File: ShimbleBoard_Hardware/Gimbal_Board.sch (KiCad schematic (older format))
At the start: 84 parts, among them Q1 Q_NMOS_GDS, Q2 Q_NMOS_GDS, Q3 Q_NMOS_GDS, Q4 Q_NMOS_GDS, Q5 Q_NMOS_GDS, Q6 Q_NMOS_GDS, Q7 Q_NMOS_GDS, Q8 Q_NMOS_GDS, SW1 SW_Push, SW10 SW_SPDT, SW2 SW_Push, SW3 SW_Push, SW4 SW_Push, SW5 SW_Push, SW6 SW_Push, SW7 SW_Push, SW8 SW_Push, SW9 SW_Push, U1 TM4C129E_Launchpad, U2 OKI, U3 OKI

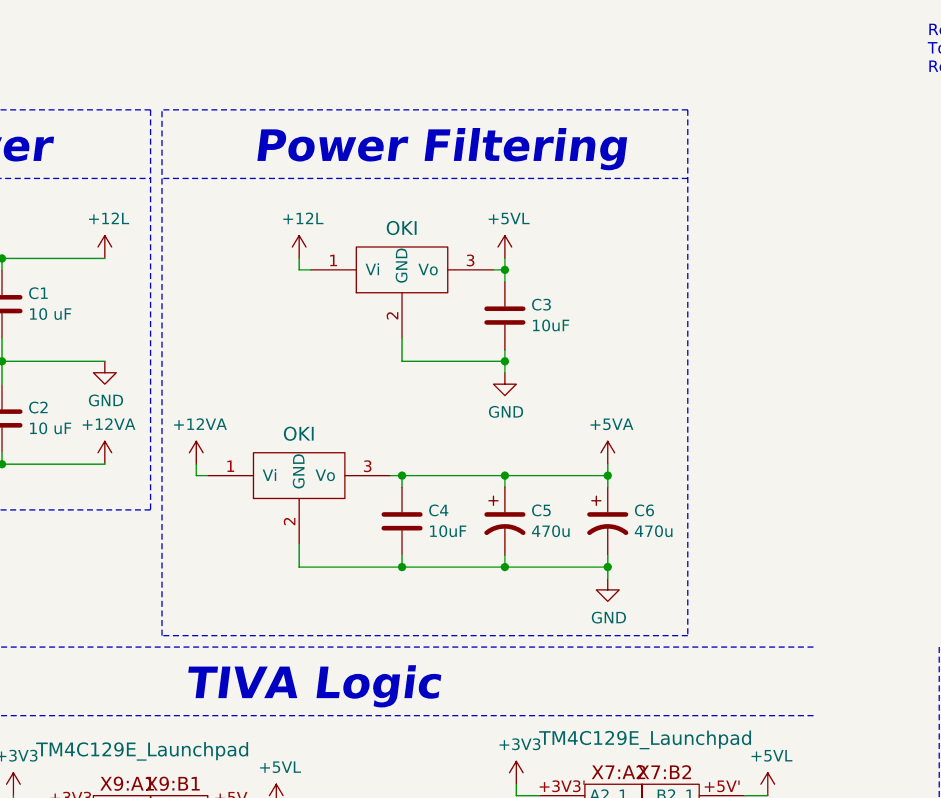
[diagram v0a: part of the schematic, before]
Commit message: Cleaned some stuff
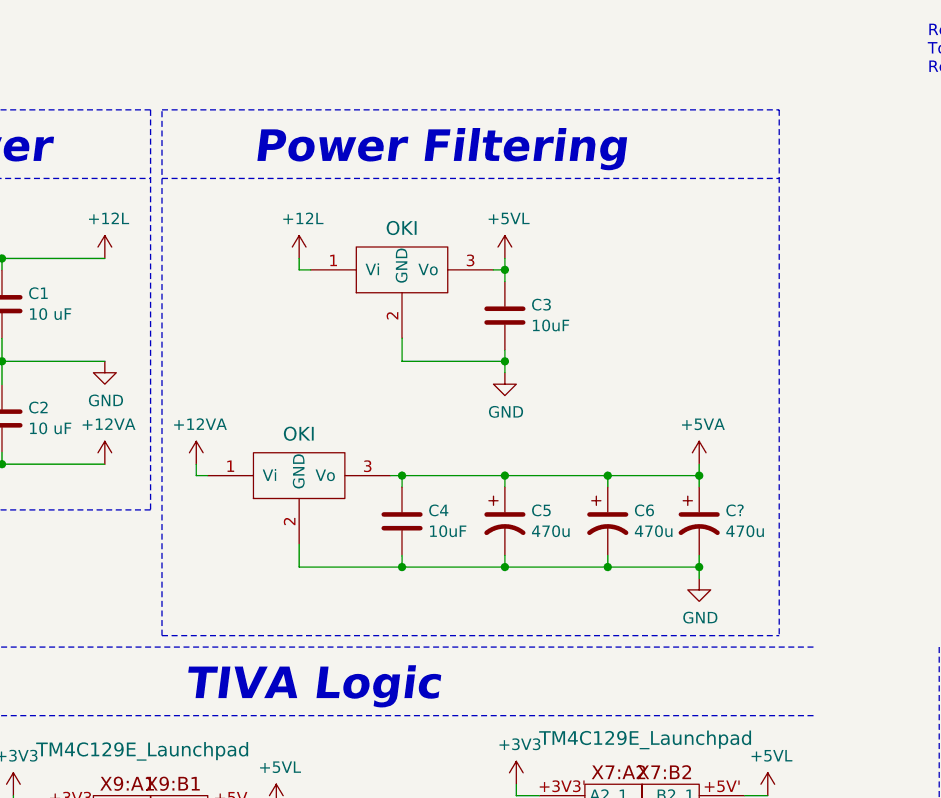
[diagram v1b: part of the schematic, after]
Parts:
- added C?: 470u, Capacitor_THT:CP_Radial_D8.0mm_P3.50mm, symbol Device:CP1
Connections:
- net +5VA: now also C?.1
- net GND: now also C?.2
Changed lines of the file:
@@
 Comment4 ""
 $EndDescr
-Connection ~ 3850 2100
-Wire Wire Line
-	3850 2050 3850 2100
 Connection ~ 3850 2500
 Wire Wire Line
-	3850 2500 3850 2550
+	4250 2500 4250 2550
 Connection ~ 2950 2500
 Wire Wire Line
@@
 Wire Wire Line
 	3850 2450 3850 2500
-Connection ~ 3400 2100
-Wire Wire Line
-	3850 2100 3850 2150
-Wire Wire Line
-	3400 2100 3850 2100
 Connection ~ 2950 2100
 Wire Wire Line
@@
 L power:+5VA #PWR07
 U 1 1 5DAD4728
-P 3850 2050
-F 0 "#PWR07" H 3850 1900 50  0001 C CNN
-F 1 "+5VA" H 3865 2223 50  0000 C CNN
-F 2 "" H 3850 2050 50  0001 C CNN
-F 3 "" H 3850 2050 50  0001 C CNN
-	1    3850 2050
-	1    0    0    -1
-$EndComp
-$Comp
-L power:GND #PWR08
-U 1 1 5DAD3C4F
-P 3850 2550
-F 0 "#PWR08" H 3850 2300 50  0001 C CNN
-F 1 "GND" H 3855 2377 50  0000 C CNN
-F 2 "" H 3850 2550 50  0001 C CNN
-F 3 "" H 3850 2550 50  0001 C CNN
-	1    3850 2550
+P 4250 2050
+F 0 "#PWR07" H 4250 1900 50  0001 C CNN
+F 1 "+5VA" H 4265 2223 50  0000 C CNN
+F 2 "" H 4250 2050 50  0001 C CNN
+F 3 "" H 4250 2050 50  0001 C CNN
+	1    4250 2050
 	1    0    0    -1
 $EndComp
@@
 $EndComp
 Wire Notes Line
-	4200 500  4200 2800
+	4600 500  4600 2800
 Text Notes 7350 7500 0    69   ~ 14
 Shimble Board
@@
 	500  800  1850 800
 Wire Notes Line
-	4200 500  1900 500
-Wire Notes Line
-	4200 2800 1900 2800
-Wire Notes Line
 	1900 2800 1900 500
-Wire Notes Line
-	4200 800  1900 800
 Text Notes 17300 7500 0    50   ~ 0
 Orange
@@
 Text GLabel 4400 11550 2    50   Output ~ 0
 Servo_SW_8
+Wire Wire Line
+	4250 2450 4250 2500
+$Comp
+L Device:CP1 C?
+U 1 1 5DD2ACC6
+P 4250 2300
+F 0 "C?" H 4365 2346 50  0000 L CNN
+F 1 "470u" H 4365 2255 50  0000 L CNN
+F 2 "Capacitor_THT:CP_Radial_D8.0mm_P3.50mm" H 4250 2300 50  0001 C CNN
+F 3 "~" H 4250 2300 50  0001 C CNN
+	1    4250 2300
+	1    0    0    -1
+$EndComp
+Connection ~ 3400 2100
+Wire Wire Line
+	3400 2100 3850 2100
+Wire Wire Line
+	3850 2100 3850 2150
+Wire Wire Line
+	4250 2050 4250 2100
+Connection ~ 3850 2100
+Wire Wire Line
+	4250 2100 4250 2150
+Wire Wire Line
+	4250 2100 3850 2100
+Wire Wire Line
+	4250 2500 3850 2500
+Connection ~ 4250 2100
+$Comp
+L power:GND #PWR08
+U 1 1 5DAD3C4F
+P 4250 2550
+F 0 "#PWR08" H 4250 2300 50  0001 C CNN
+F 1 "GND" H 4255 2377 50  0000 C CNN
+F 2 "" H 4250 2550 50  0001 C CNN
+F 3 "" H 4250 2550 50  0001 C CNN
+	1    4250 2550
+	1    0    0    -1
+$EndComp
+Connection ~ 4250 2500
+Wire Notes Line
+	1900 2800 4600 2800
+Wire Notes Line
+	1900 800  4600 800
+Wire Notes Line
+	1900 500  4600 500
 $EndSCHEMATC

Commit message: Cleaned
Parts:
- gave numbers to parts that had none: 1
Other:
- note added: "Servo Buttons"
- note added: "Servo Switches"
- moved on the sheet: C1, C2, C3, C4, C5, C6, C7, Conn1, Conn2, Conn3, Conn4, Conn5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
